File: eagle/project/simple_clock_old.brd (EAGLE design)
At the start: 75.5 x 70.7 mm, 10 parts, among them U1 STM32F103C8T6, U2 MAX7219CNG, U3 AMS1117_50_REG

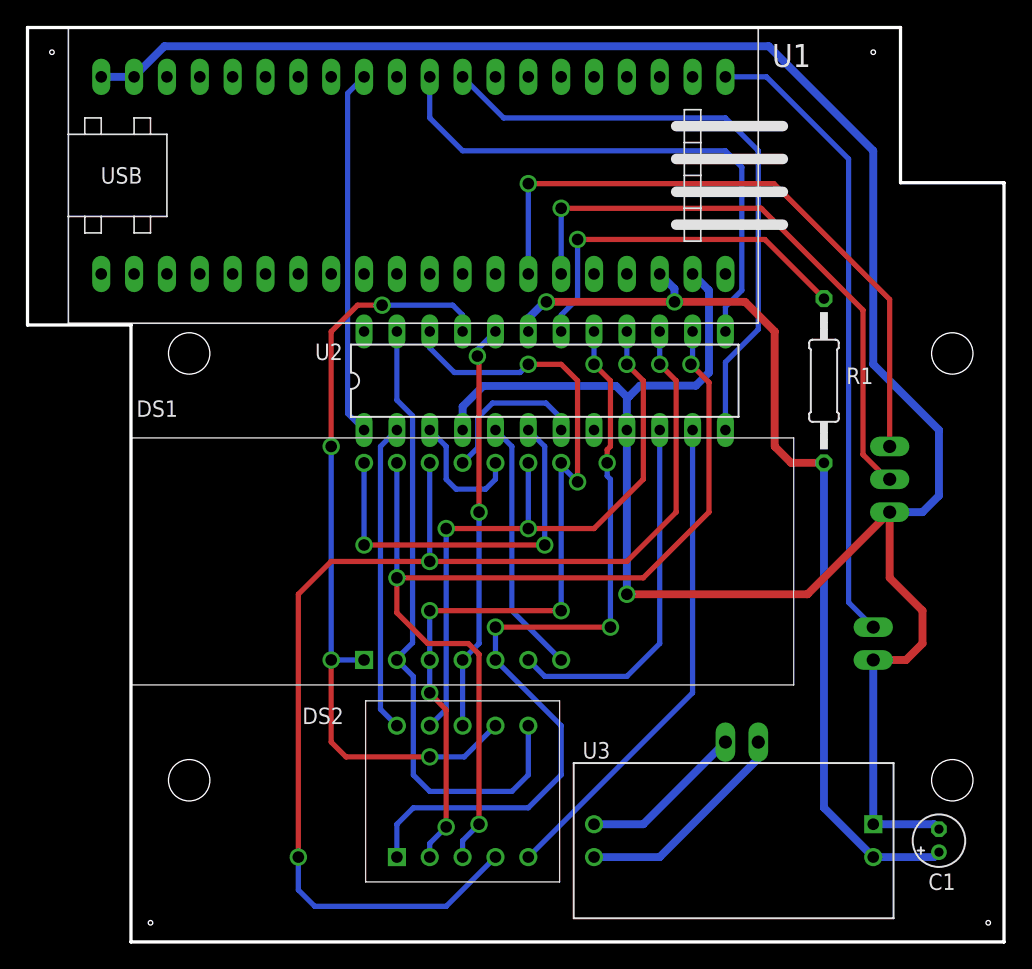
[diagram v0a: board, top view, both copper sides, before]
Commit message: revised pcb
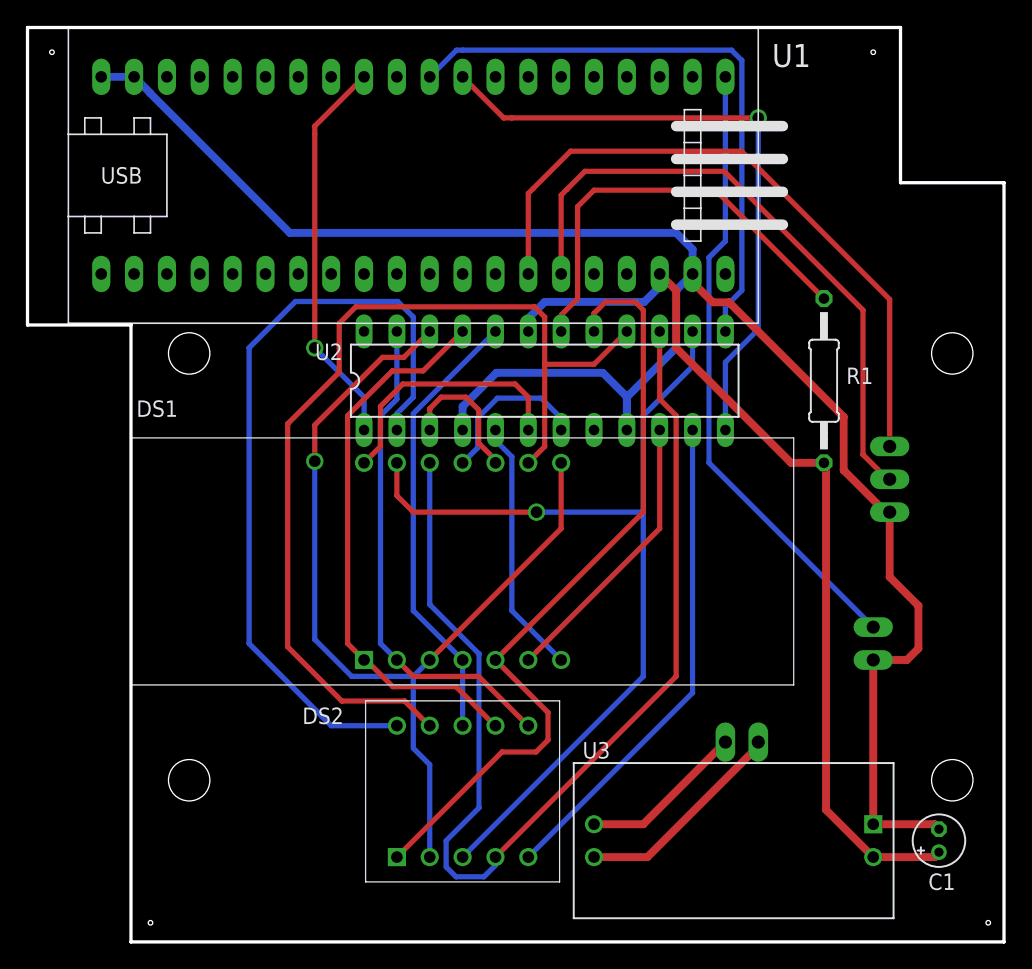
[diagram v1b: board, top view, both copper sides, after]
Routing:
- net GND: track 199.6 -> 145.2 mm, vias 1 -> 0
- net N$5: track 23.9 -> 60.9 mm
- net N$25: track 49.6 -> 76.1 mm, vias 3 -> 0
- net N$12: track 61.0 -> 43.3 mm, vias 4 -> 0
- net N$16: track 49.6 -> 38.7 mm
- net N$4: track 29.7 -> 20.0 mm, vias 2 -> 0
- net N$14: track 94.2 -> 86.0 mm, vias 3 -> 0
- net N$17: track 65.8 -> 73.0 mm, vias 6 -> 1
- net N$8: track 28.2 -> 22.0 mm
- net N$11: track 76.3 -> 70.1 mm, vias 3 -> 1
- net N$9: track 42.1 -> 46.8 mm
- net N$19: track 28.6 -> 33.2 mm, vias 1 -> 0
- net N$15: track 31.6 -> 34.7 mm, vias 2 -> 0
- net N$21: track 45.7 -> 48.7 mm, vias 1 -> 0
- net +5V: track 74.7 -> 71.9 mm, vias 2 -> 0
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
